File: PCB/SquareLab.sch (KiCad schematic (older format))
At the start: 12 parts

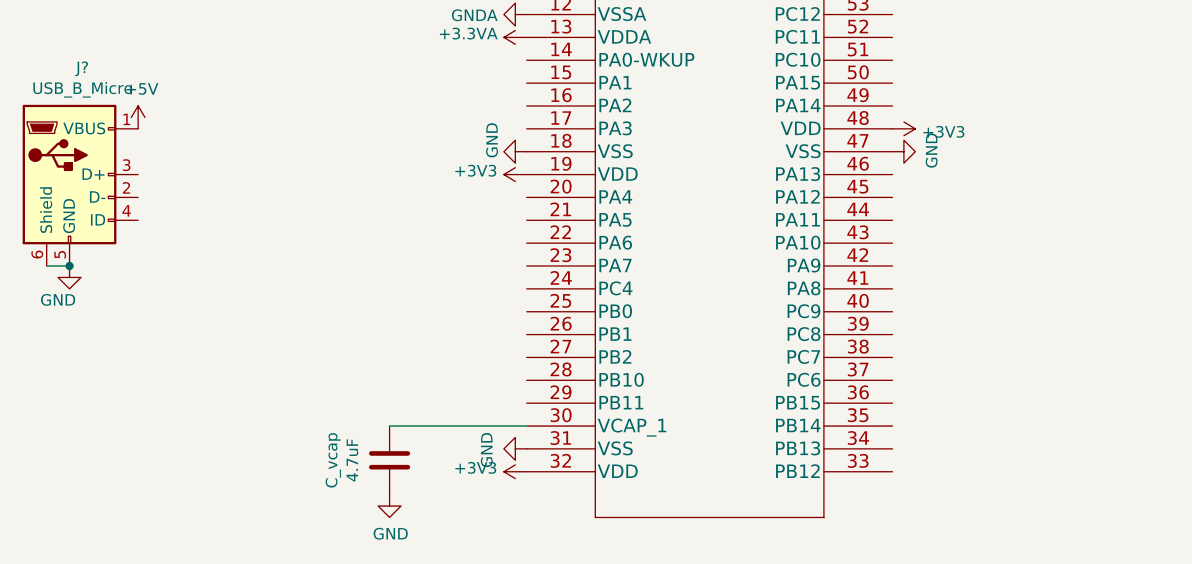
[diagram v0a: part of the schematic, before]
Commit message: Some updates schematic side
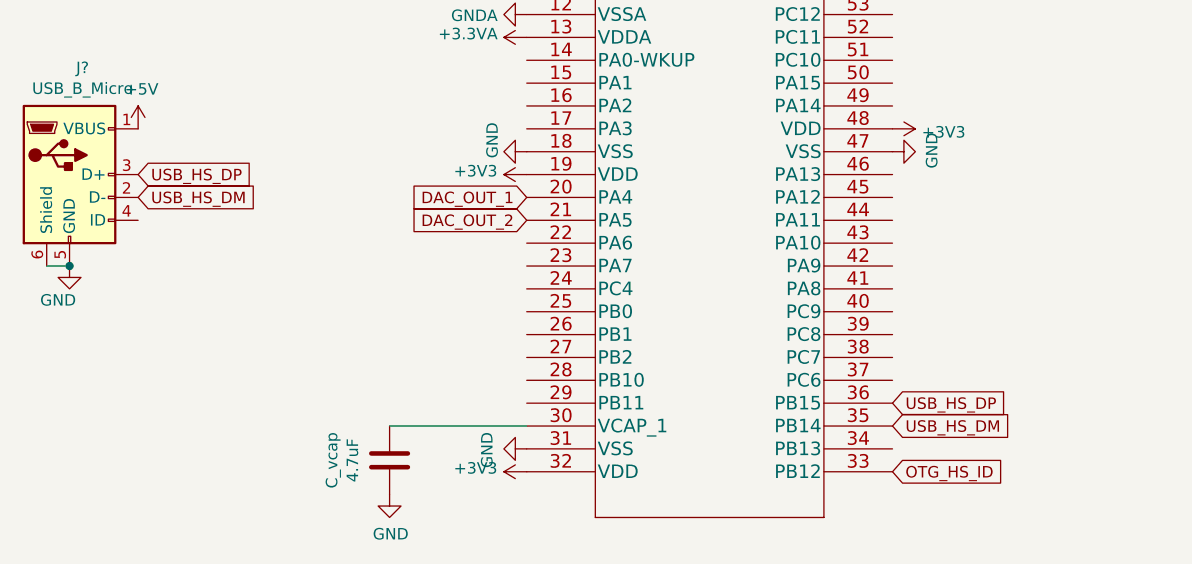
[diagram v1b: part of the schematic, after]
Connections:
- net DAC_OUT_1: now reaches U?.20 (PA4)
- net DAC_OUT_2: now reaches U?.21 (PA5)
- net OTG_HS_ID: now reaches U?.33 (PB12)
- net USB_HS_DM: now reaches U?.35 (PB14)
- net USB_HS_DM: now also J?.2 (D-)
- net USB_HS_DP: now reaches U?.36 (PB15)
- net USB_HS_DP: now also J?.3 (D+)
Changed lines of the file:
@@
 	1450 5400 1550 5400
 Connection ~ 1550 5400
+Text GLabel 3550 5100 0    50   Input ~ 0
+DAC_OUT_1
+Text GLabel 3550 5200 0    50   Input ~ 0
+DAC_OUT_2
+Text GLabel 5150 6000 2    50   Input ~ 0
+USB_HS_DP
+Text GLabel 5150 6100 2    50   Input ~ 0
+USB_HS_DM
+Text GLabel 1850 5000 2    50   Input ~ 0
+USB_HS_DP
+Text GLabel 1850 5100 2    50   Input ~ 0
+USB_HS_DM
+Text GLabel 5150 6300 2    50   Input ~ 0
+OTG_HS_ID
 $EndSCHEMATC

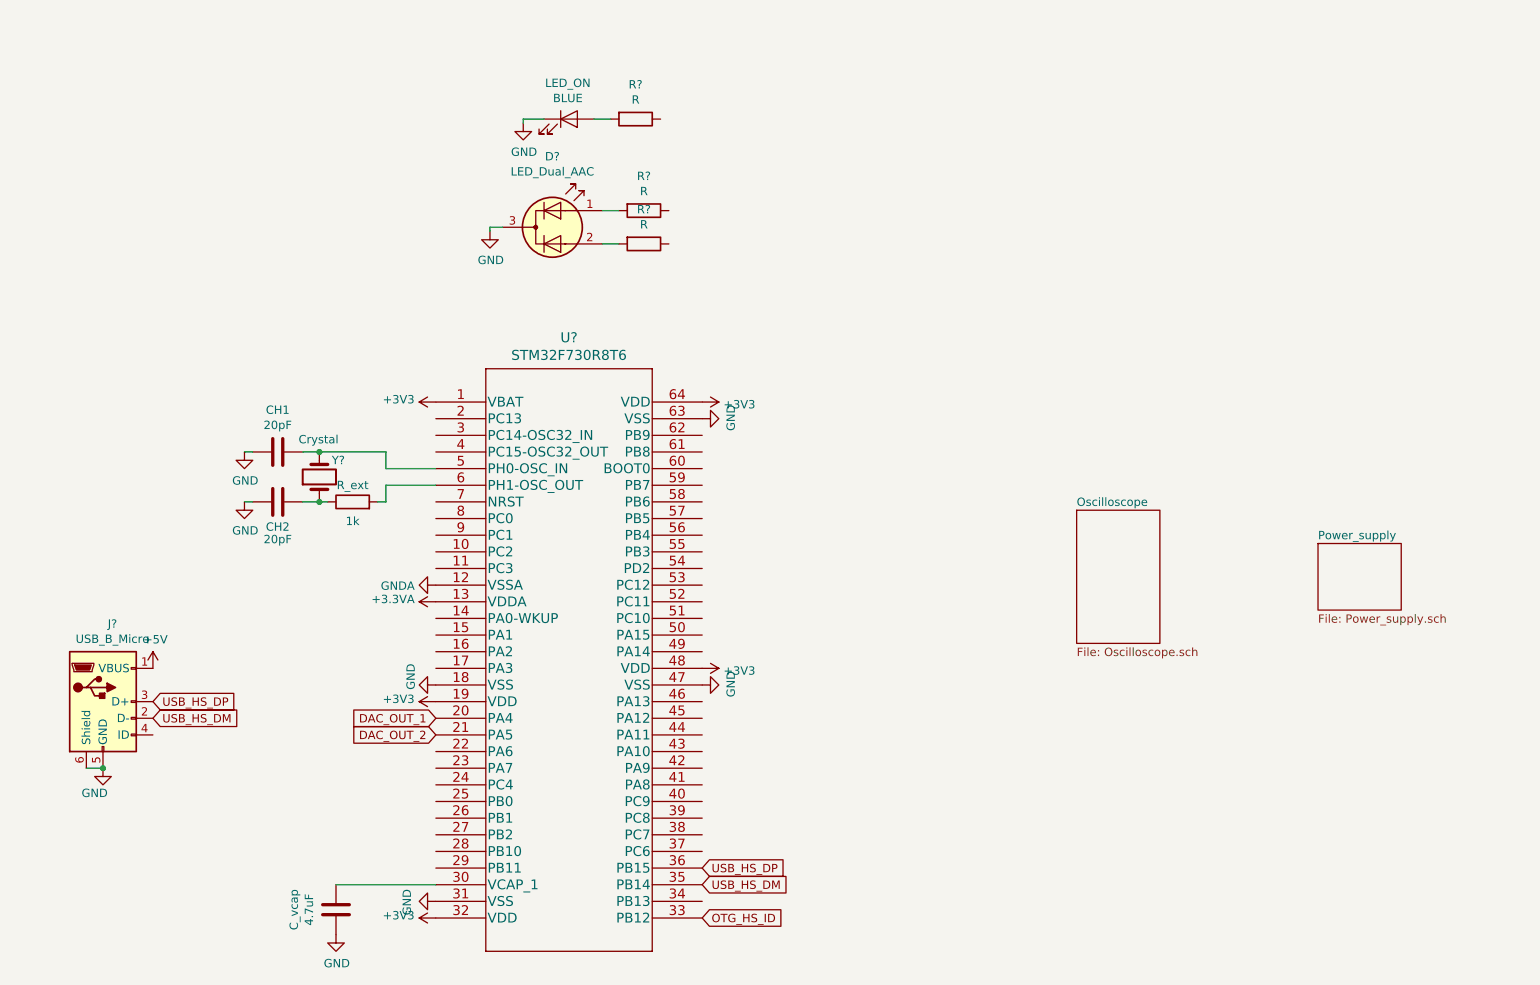
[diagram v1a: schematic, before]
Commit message: Advancing in the schmatic. Power to be finished
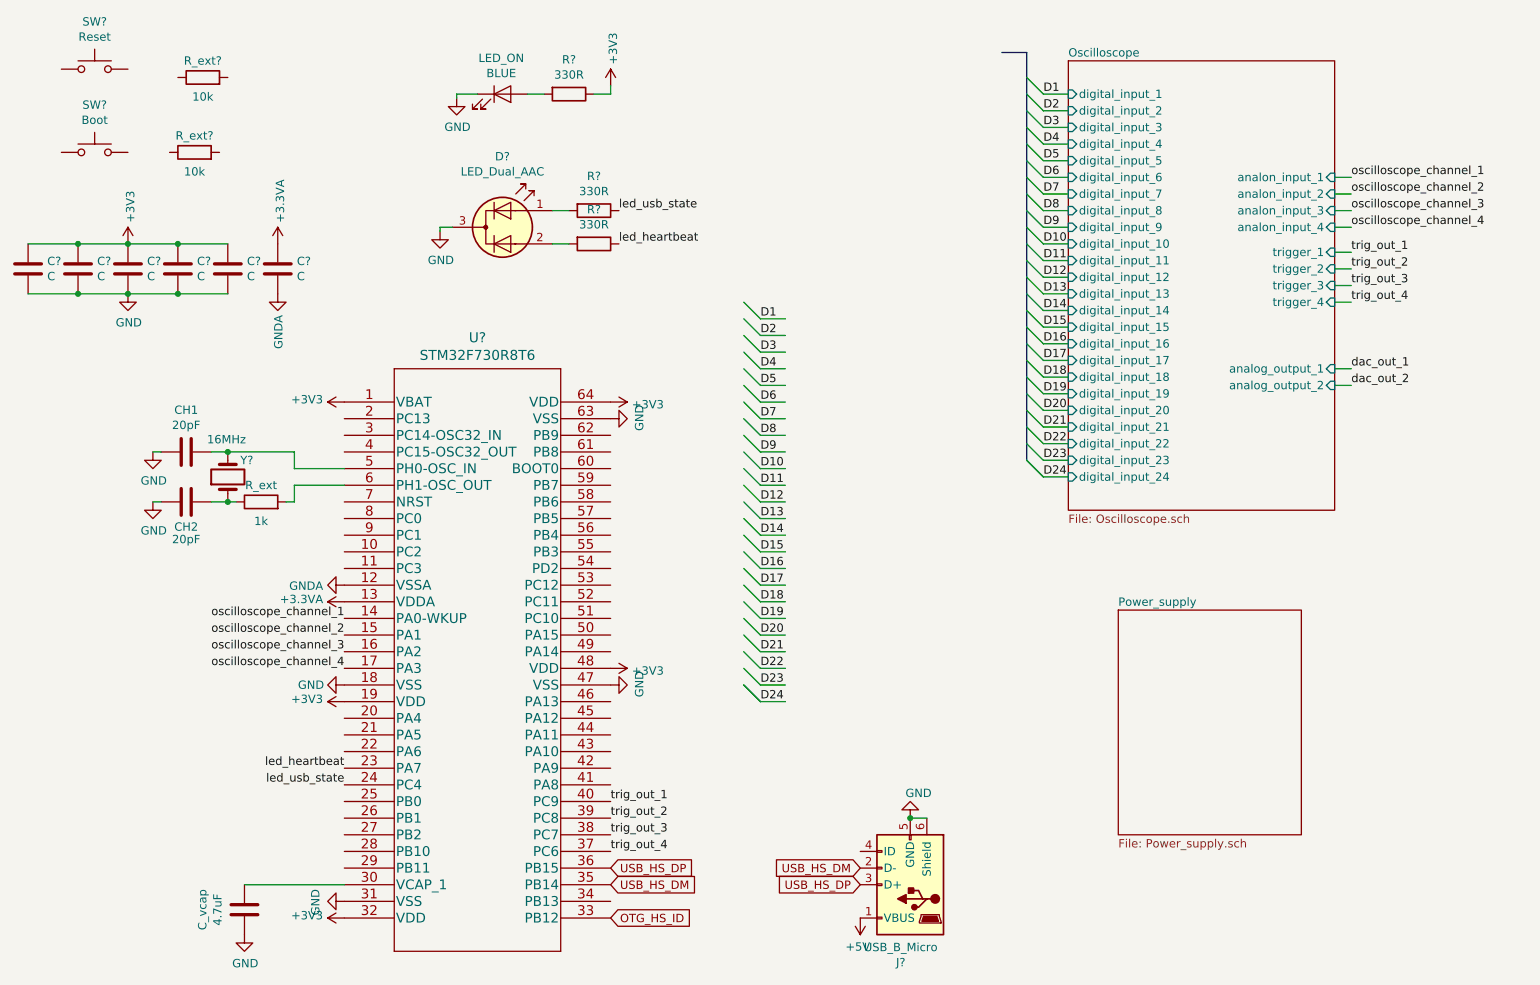
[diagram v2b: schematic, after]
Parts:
- added C? (x6): C, symbol Device:C
- added R_ext? (x2): 10k, symbol Device:R
- added SW?: Reset, symbol Switch:SW_Push
- added SW?: Boot, symbol Switch:SW_Push
- R? (x3): value R -> 330R
- Y?: value Crystal -> 16MHz
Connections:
- net labels added: D1, D10, D11, D12, D13, D14, D15, D16, D17, D18, D19, D2, D20, D21, D22, D23, D24, D3, D4, D5, D6, D7, D8, D9, dac_out_1, dac_out_2, led_heartbeat, led_usb_state, oscilloscope_channel_1, oscilloscope_channel_2, oscilloscope_channel_3, oscilloscope_channel_4, trig_out_1, trig_out_2, trig_out_3, trig_out_4
- net labels removed: DAC_OUT_1, DAC_OUT_2
- wire segments 20 -> 88
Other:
- moved on the sheet: CH1, CH2, C_vcap, D?, J?, LED_ON, R?, R_ext, U?, Y?
